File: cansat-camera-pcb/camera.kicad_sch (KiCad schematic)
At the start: 17 parts, among them IC2 TLV74315PDBVR, J6 OV5640, U6 TLV74328PDBVR

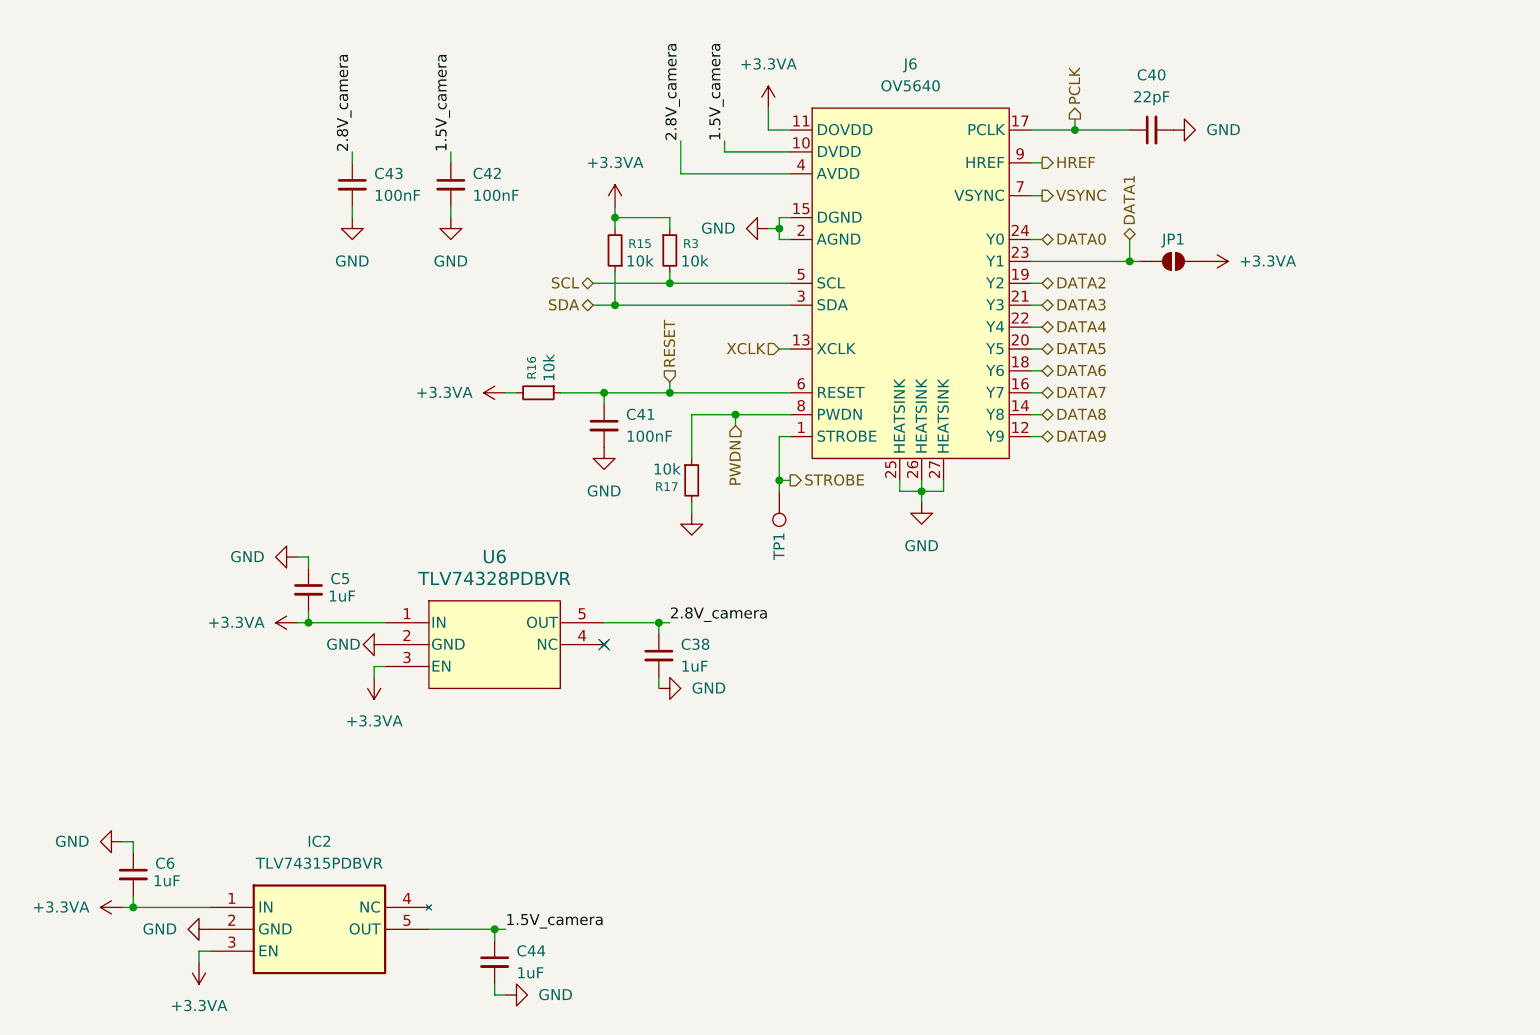
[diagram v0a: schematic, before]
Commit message: milan eszi a havat(unicummal)  (jonas is zabalja)
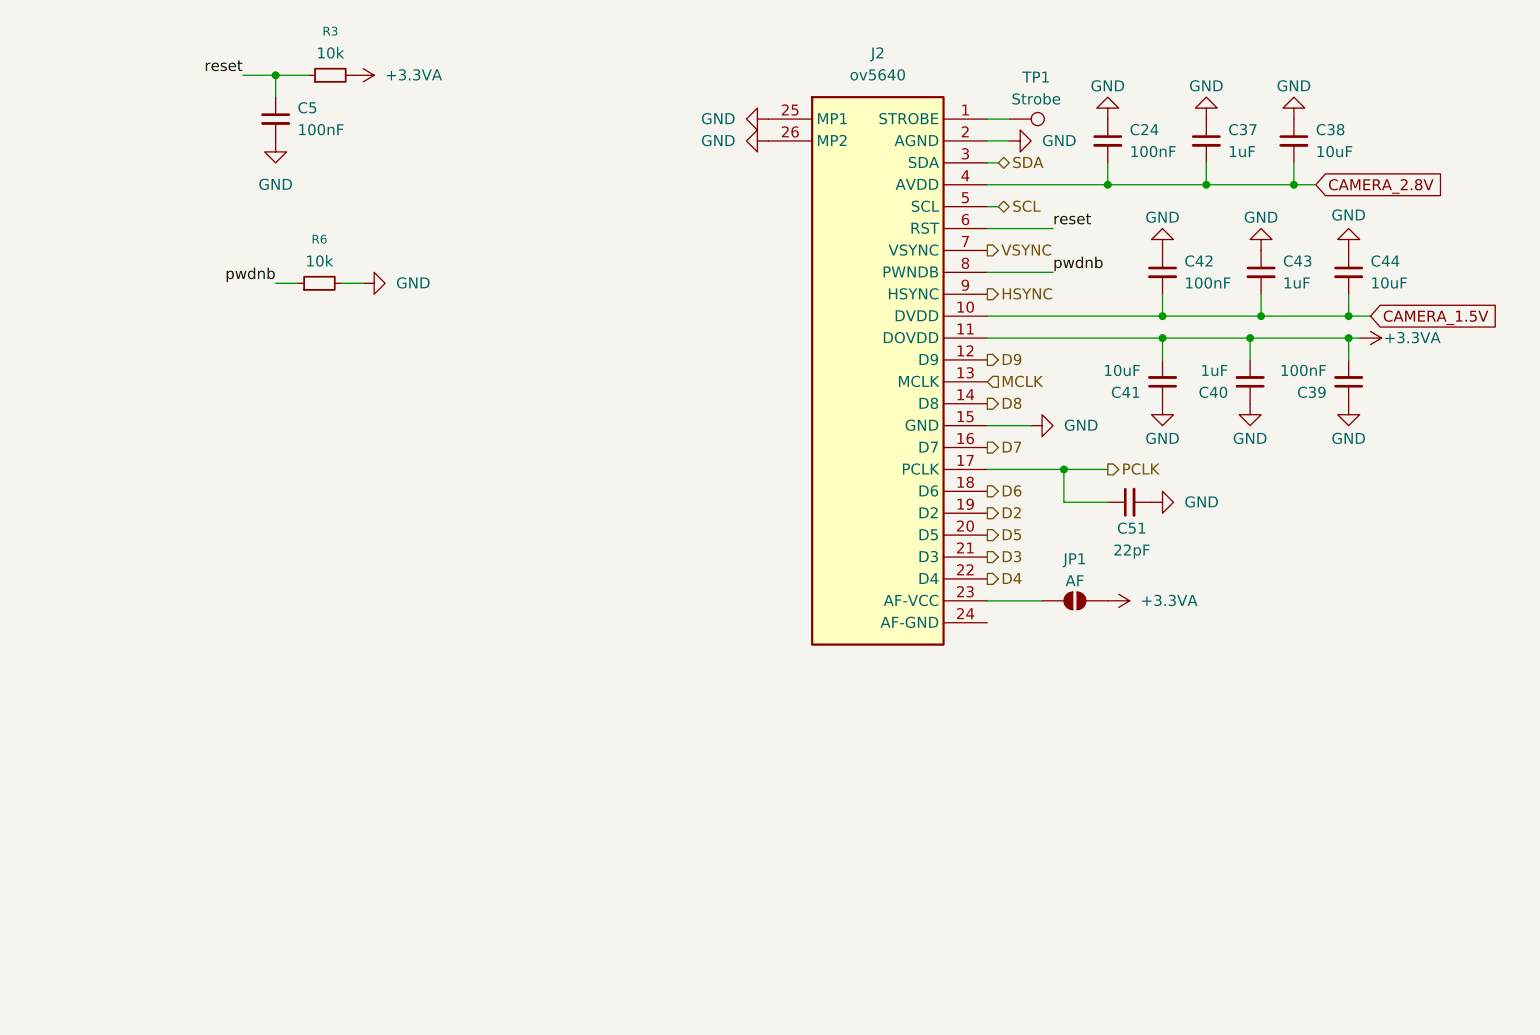
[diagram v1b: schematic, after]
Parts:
- removed C6: 1uF, Capacitor_SMD:C_0603_1608Metric, symbol Device:C_Small
- removed IC2: TLV74315PDBVR, gaia-camera-footprints:TLV74315PDBVR, symbol gaia-camera-symbols:TLV74315PDBVR
- removed J6: OV5640, gaia-camera-footprints:OV5640, symbol gaia-camera-symbols:OV2640
- removed R15, R16, R17: 10k, Resistor_SMD:R_0402_1005Metric, symbol Device:R_Small
- removed U6: TLV74328PDBVR, gaia-camera-footprints:TLV74328PDBVR, symbol gaia-camera-symbols:TLV74328PDBVR
- added C24, C39: 100nF, Capacitor_SMD:C_0402_1005Metric, symbol Device:C_Small
- added C37: 1uF, Capacitor_SMD:C_0603_1608Metric, symbol Device:C_Small
- added C51: 22pF, Capacitor_SMD:C_0402_1005Metric, symbol Device:C_Small
- added J2: ov5640, gaia-camera-footprints:F33Z1A7Q1E8C24, symbol gaia-camera-symbols:ov5640
- added R6: 10k, Resistor_SMD:R_0402_1005Metric, symbol Device:R_Small
- C38, C44: value 1uF -> 10uF
- C40: value 22pF -> 1uF; footprint Capacitor_SMD:C_0402_1005Metric -> Capacitor_SMD:C_0603_1608Metric
- C41: value 100nF -> 10uF; footprint Capacitor_SMD:C_0402_1005Metric -> Capacitor_SMD:C_0603_1608Metric
- C43: value 100nF -> 1uF; footprint Capacitor_SMD:C_0402_1005Metric -> Capacitor_SMD:C_0603_1608Metric
- C5: value 1uF -> 100nF; footprint Capacitor_SMD:C_0603_1608Metric -> Capacitor_SMD:C_0402_1005Metric
- JP1: value SolderJumper_2_Open -> AF
- TP1: value TestPoint -> Strobe; footprint TestPoint:TestPoint_Pad_2.0x2.0mm -> TestPoint:TestPoint_Pad_1.5x1.5mm
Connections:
- net 1.5V_camera is gone; now on net GND: C42.1, C44.1
- net 2.8V_camera is gone; now on net GND: C38.1, C43.1
- net RESET is gone; now on net GND: C41.1
- net +3.3VA: now also C40.2, C41.2, R3.2, C39.2, J2.11 (DOVDD); no longer C5.2, R3.1
- net GND: now also C40.1, C5.2, C24.1, C37.1, C39.1, C51.2, J2.15 (GND), J2.2 (AGND), J2.25 (MP1), J2.26 (MP2), R6.2; no longer C38.2, C40.2, C41.2, C42.2, C43.2, C44.2, C5.1
- net PCLK: now also C51.1, J2.17 (PCLK); no longer C40.1
- net SCL: now also J2.5 (SCL); no longer R3.2
- net SDA: now also J2.3 (SDA)
- net VSYNC: now also J2.7 (VSYNC)
- net DATA1: no longer names the net of JP1.1 (A)
- net DATA1: now also J2.23 (AF-VCC)
- net STROBE: no longer names the net of TP1.1
- net STROBE: now also J2.1 (STROBE)
- new net CAMERA_1.5V: C42.2, C43.2, C44.2, J2.10 (DVDD)
- new net CAMERA_2.8V: C24.2, C37.2, C38.2, J2.4 (AVDD)
- new net D2: J2.19 (D2)
- new net D3: J2.21 (D3)
- new net D4: J2.22 (D4)
- new net D5: J2.20 (D5)
- new net D6: J2.18 (D6)
- new net D7: J2.16 (D7)
- new net D8: J2.14 (D8)
- new net D9: J2.12 (D9)
- new net HSYNC: J2.9 (HSYNC)
- new net MCLK: J2.13 (MCLK)
- new net pwdnb: J2.8 (PWNDB), R6.1
- new net reset: C5.1, J2.6 (RST), R3.1
- no-connect marks 1 -> 0
